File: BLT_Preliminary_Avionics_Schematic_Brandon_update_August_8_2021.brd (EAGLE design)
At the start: 144.8 x 55.5 mm, 30 parts, among them Y1 32.768kHz

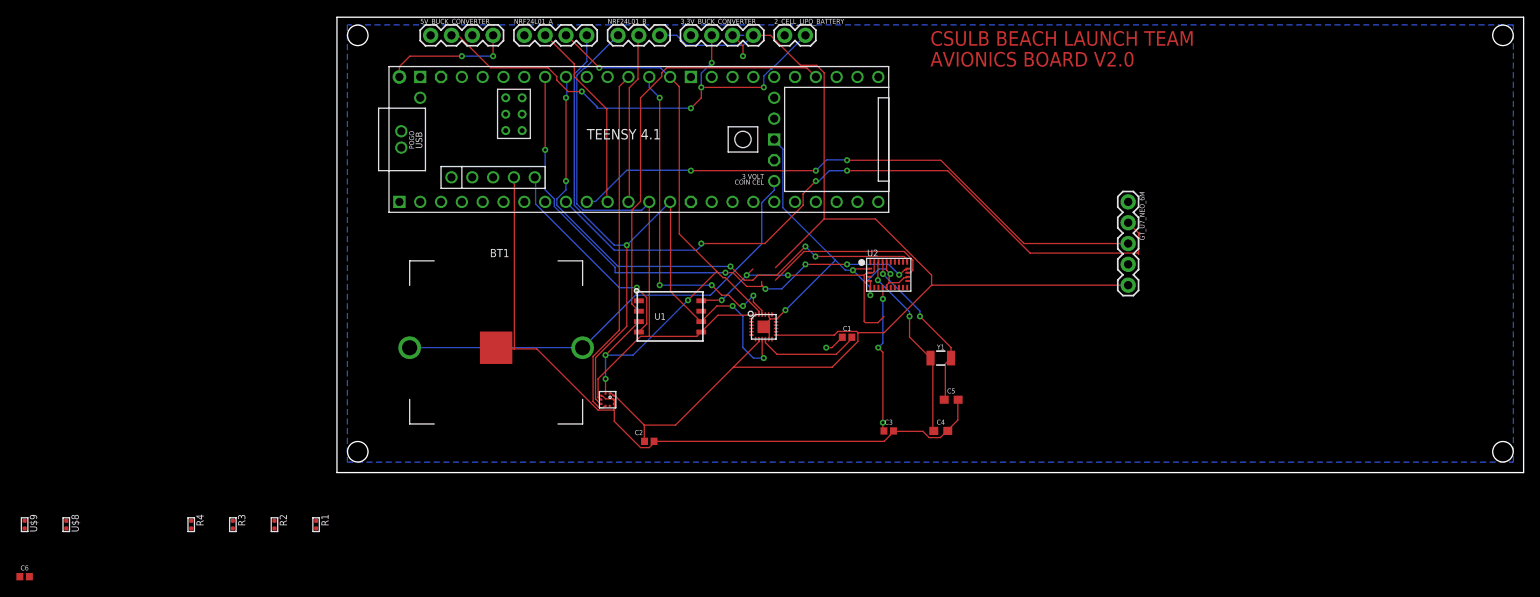
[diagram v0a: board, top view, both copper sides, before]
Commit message: Updated files
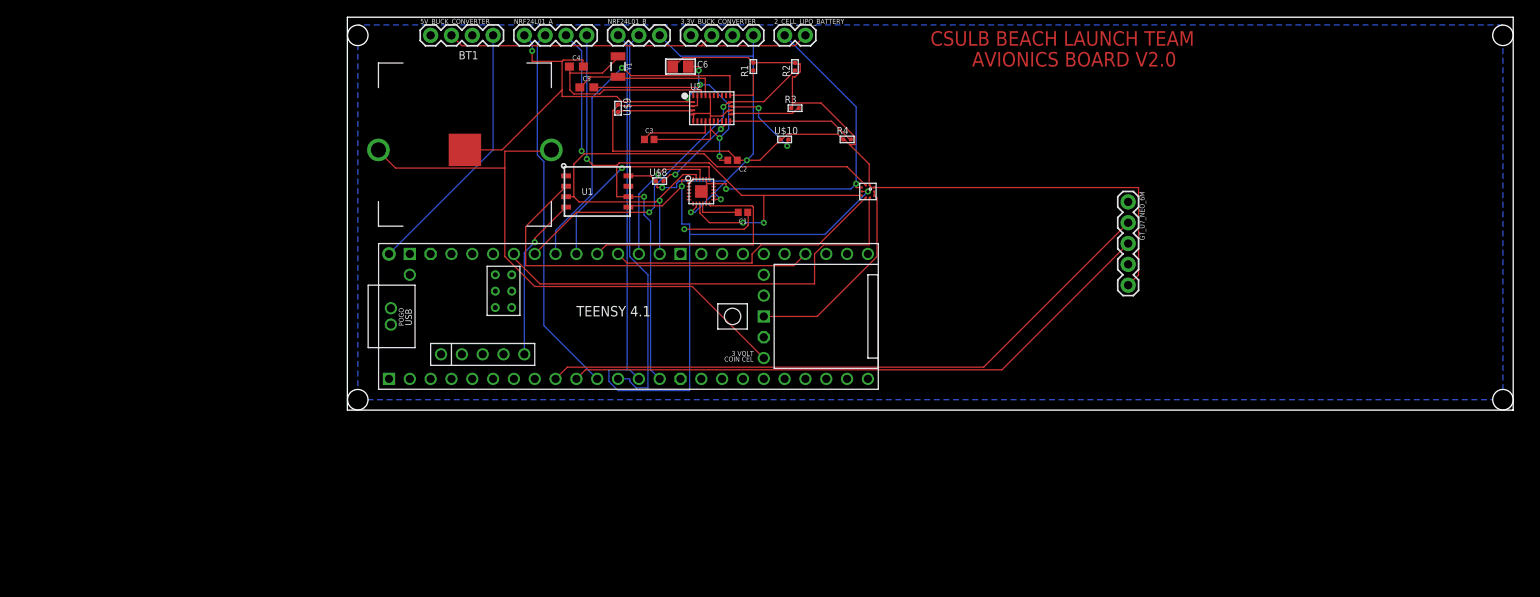
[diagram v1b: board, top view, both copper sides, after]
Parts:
- added U$10: 10K, OPL_Resistor:R0402
- C6: value 470nF -> 47uF; device SparkFun-Capacitors:0402 -> microbuilder:0805
- moved C6 101.4 mm to (41.9, 49.5)
- moved R4 92.8 mm to (62.2, 40.6), turned to 90 degrees
- moved U$9 88.4 mm to (34.3, 44.5)
- moved R3 85.3 mm to (55.9, 44.5), turned to 90 degrees
- moved R2 84.6 mm to (55.9, 49.5), turned to 180 degrees
- moved U$8 83.6 mm to (39.4, 35.6), turned to 90 degrees
- moved R1 77.3 mm to (50.8, 49.5), turned to 180 degrees
- moved C4 62.9 mm to (29.2, 49.5)
- moved C5 58.5 mm to (30.5, 47.0)
- moved Y1 53.1 mm to (34.3, 49.5), turned to 270 degrees
- moved C3 46.0 mm to (38.1, 40.6)
- moved U$3 40.7 mm to (64.8, 34.3)
- moved C2 35.8 mm to (48.3, 38.1), turned to 180 degrees
- moved U2 29.6 mm to (45.7, 44.5)
- moved BT1 24.4 mm to (5.08, 39.4)
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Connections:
- net 3.3V: now also C6.1, U$10.1; no longer C6.2
- net GND: now also C6.2; no longer C6.1
- net N$5: now also U$10.2
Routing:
- net BMPINT: track 0.00 -> 55.1 mm
- net MOSI: track 74.1 -> 117.5 mm, vias 0 -> 2
- net ICMINT1: track 0.00 -> 29.7 mm
- net CSN: track 20.9 -> 48.7 mm
- net ICMINT2: track 0.00 -> 25.0 mm, vias 0 -> 1
- net CS3: track 41.7 -> 17.2 mm, vias 5 -> 1
- net SCL: track 66.7 -> 43.3 mm, vias 6 -> 2
- net CE: track 23.5 -> 45.3 mm
- net GND: track 177.3 -> 198.5 mm, vias 7 -> 10
- net SDA: track 65.4 -> 47.9 mm, vias 5 -> 1
- net 5V: track 15.8 -> 31.9 mm, vias 2 -> 0
- net N$6: track 0.00 -> 15.7 mm
- net VBAT: track 56.5 -> 71.7 mm
- net BAT+: track 59.3 -> 46.0 mm, vias 5 -> 0
- net N$7: track 0.00 -> 10.9 mm, vias 0 -> 2
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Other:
- board size 144.8 x 55.5 mm -> 142.2 x 47.9 mm

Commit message: updated files even more
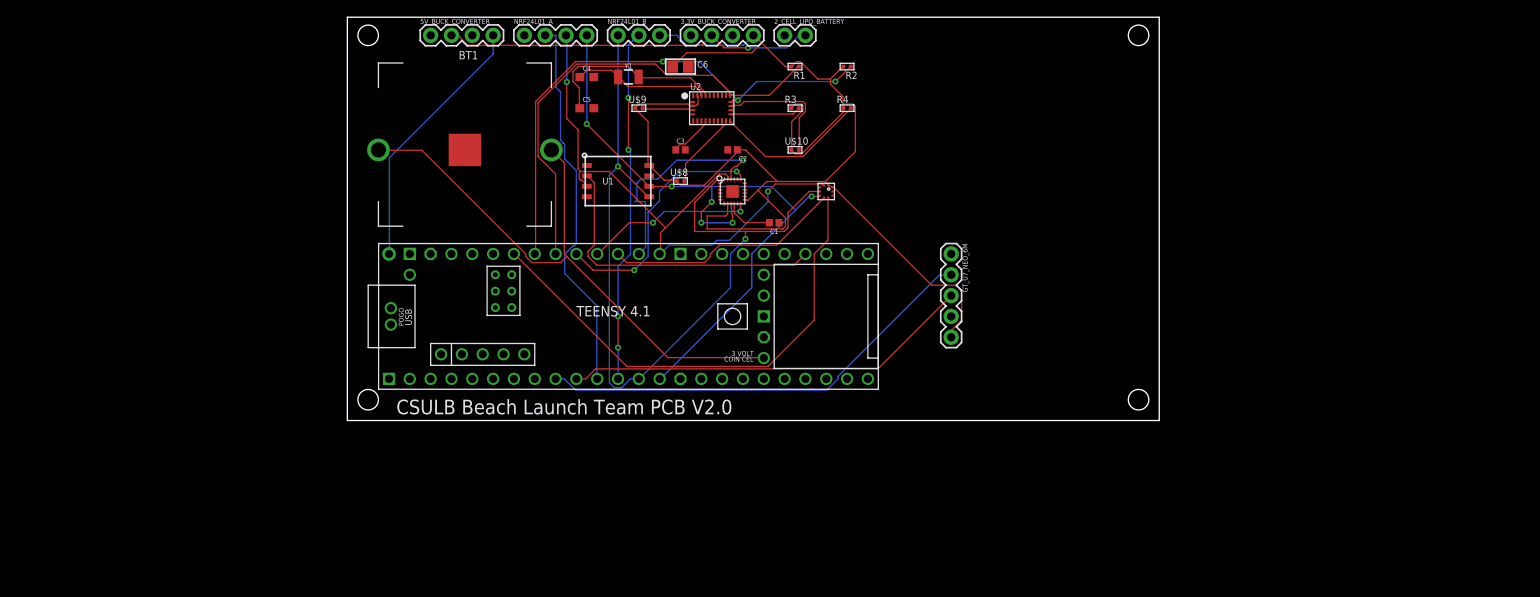
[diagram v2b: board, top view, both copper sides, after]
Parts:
- moved U$6 44.5 mm to (97.8, 8.89)
- moved U$7 44.5 mm to (97.8, 53.3)
- moved GT_U7_NEO_6M 22.5 mm to (74.9, 26.7)
- moved R2 6.35 mm to (62.2, 49.5), turned to 270 degrees
- moved R1 5.08 mm to (55.9, 49.5), turned to 270 degrees
- moved U$3 5.08 mm to (59.7, 34.3)
- moved C1 4.02 mm to (53.3, 30.5)
- moved C3 4.02 mm to (41.9, 39.4)
- moved R4 3.81 mm to (62.2, 44.5)
- moved U$2 3.81 mm to (48.3, 34.3)
- moved U1 2.84 mm to (34.3, 35.6)
- moved C5 2.54 mm to (30.5, 44.5)
- moved U$8 2.54 mm to (41.9, 35.6)
- moved U$9 2.54 mm to (36.8, 44.5), turned to 90 degrees
- moved U$10 1.80 mm to (55.9, 39.4)
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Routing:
- net GND: track 198.5 -> 0.00 mm, vias 10 -> 0
- net TX2: track 74.1 -> 49.9 mm
- net RX2: track 77.7 -> 54.8 mm
- net SCL: track 43.3 -> 63.8 mm, vias 2 -> 3
- net 3.3V: track 187.5 -> 169.9 mm, vias 4 -> 0
- net MOSI: track 117.5 -> 102.6 mm
- net MISO: track 93.6 -> 83.0 mm, vias 4 -> 6
- net CS3: track 17.2 -> 27.5 mm
- net SCK: track 81.9 -> 71.7 mm
- net N$2: track 26.8 -> 16.7 mm
- net ICMINT1: track 29.7 -> 20.6 mm, vias 0 -> 2
- net SDA: track 47.9 -> 56.4 mm, vias 1 -> 0
- net CS1: track 46.5 -> 38.1 mm
- net CS4: track 34.6 -> 29.1 mm
- net CSN: track 48.7 -> 43.2 mm, vias 0 -> 4
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- removed copper zone on layer 16, net GND
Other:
- board size 142.2 x 47.9 mm -> 99 x 49.2 mm
- board text added: "CSULB Beach Launch Team PCB V2.0"
- board text removed: "AVIONICS BOARD V2.0"
- board text removed: "CSULB BEACH LAUNCH TEAM"
